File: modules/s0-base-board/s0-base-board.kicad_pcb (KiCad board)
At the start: 2 copper layers, 54.6 x 86.4 mm, 64 parts, among them J1 USB_C_Receptacle_USB2.0_14P, J2 Screw_Terminal_01x02, J3 BAT_JST_01x02, J4 RJ45_Bel_SI-60062-F JLC(C3467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, J5 Conn_02x23_Odd_Even, J6 Conn_02x23_Odd_Even, Q1 PMOS, U1 MCP73831-2-OT, U2 XL1509-5.0, U3 LM2575-3.3BU, U4 W5500, U5 NUP4202, Y1 25MHz

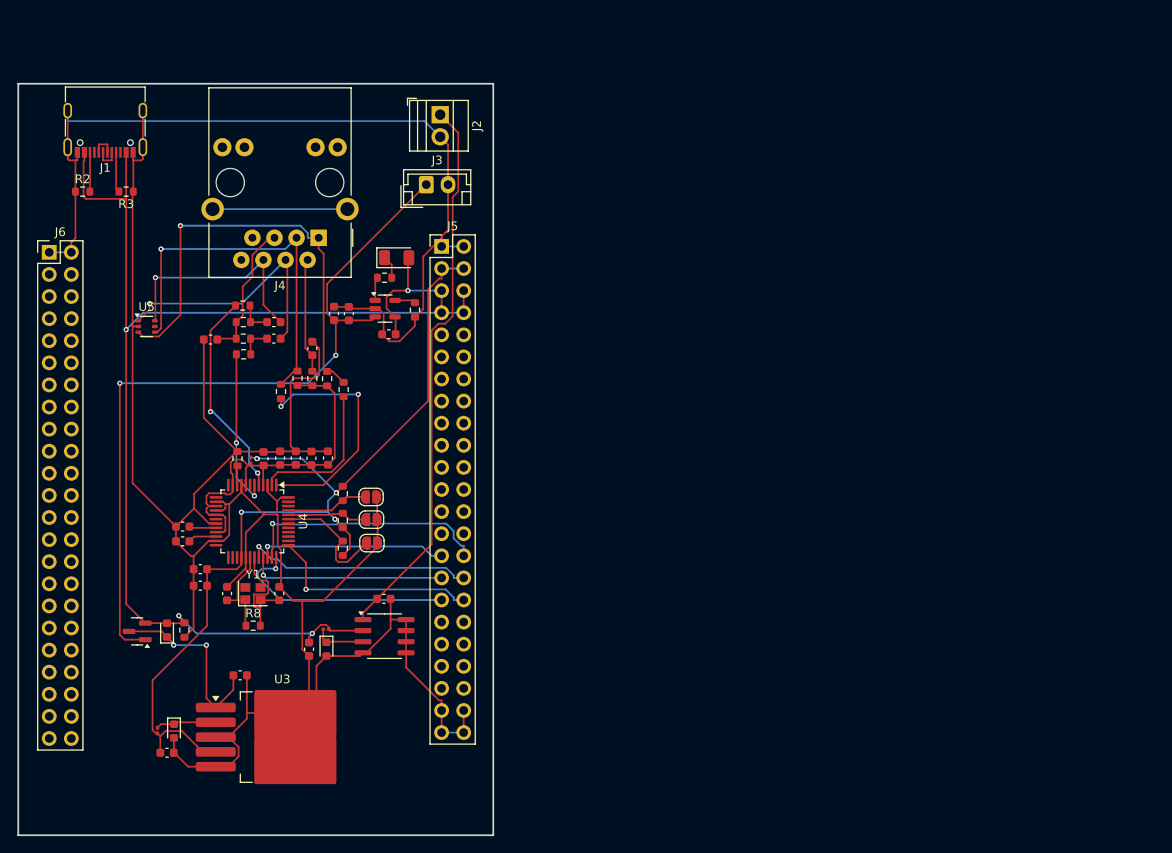
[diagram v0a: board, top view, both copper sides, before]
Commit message: Production build
Signed-off-by: Rodney Osodo <socials@rodneyosodo.com>
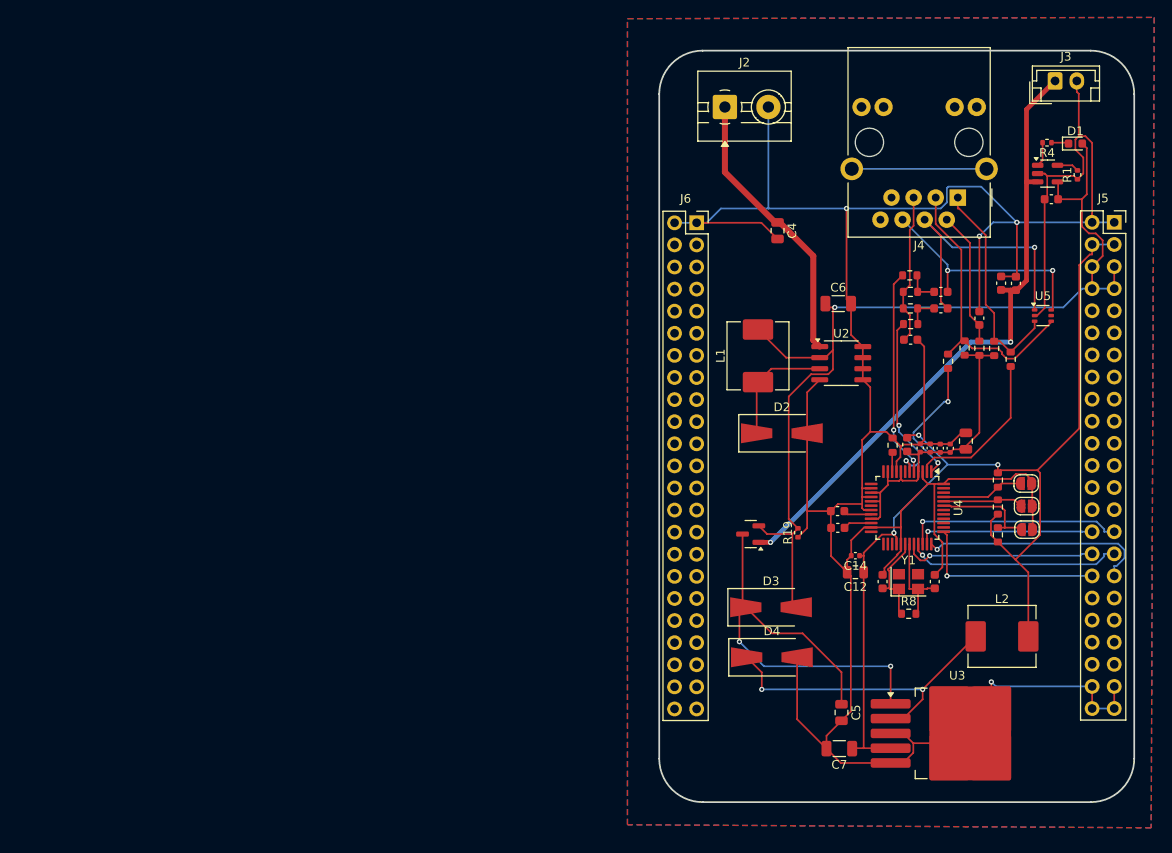
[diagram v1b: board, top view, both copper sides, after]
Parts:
- removed J1: USB_C_Receptacle_USB2.0_14P, Connector_USB:USB_C_Receptacle_G-Switch_GT-USB-7010ASV
- removed R2, R3: 5K1, Resistor_SMD:R_0603_1608Metric
- C10, C13, C14, C9: footprint Capacitor_SMD:C_0603_1608Metric -> Capacitor_SMD:C_0402_1005Metric
- C12: footprint Capacitor_SMD:C_0603_1608Metric -> Capacitor_SMD:C_0805_2012Metric
- C16: value 4.7uF -> 0.1uF; footprint Capacitor_SMD:C_0603_1608Metric -> Capacitor_SMD:C_0402_1005Metric
- C17: value 10nF -> 4.7uF
- C21: value 0.1uF -> 10uF; footprint Capacitor_SMD:C_0603_1608Metric -> Capacitor_SMD:C_0805_2012Metric
- C22: value 10uF -> 10nF
- C4, C5: value 680uF -> 10uF; footprint Capacitor_SMD:C_0603_1608Metric -> Capacitor_SMD:C_0805_2012Metric
- C6, C7: footprint Capacitor_SMD:C_0603_1608Metric -> Capacitor_SMD:C_1206_3216Metric
- D1: footprint LED_SMD:LED_1206_3216Metric -> LED_SMD:LED_0603_1608Metric
- D2, D3, D4: value D -> 40V 3A 550mV@3A Schottky; footprint Diode_SMD:D_0603_1608Metric -> Diode_SMD:D_SMA-SMB_Universal_Handsoldering
- J2: footprint TerminalBlock:TerminalBlock_Xinya_XY308-2.54-2P_1x02_P2.54mm_Horizontal -> TerminalBlock:TerminalBlock_MaiXu_MX126-5.0-02P_1x02_P5.00mm
- J4: value RJ45_Bel_SI-60062-F JLC(C34677) -> RJ45_Bel_SI-60062-F JLC
- J5, J6: footprint Connector_PinHeader_2.54mm:PinHeader_2x23_P2.54mm_Vertical -> Connector_PinSocket_2.54mm:PinSocket_2x23_P2.54mm_Vertical
- L1: value 68uH/2A -> 47uH/2A; footprint Inductor_SMD:L_0201_0603Metric -> Inductor_SMD:L_Chilisin_BMRB00060624
- L2: value 33uH -> 47uH/2A; footprint Inductor_SMD:L_0201_0603Metric -> Inductor_SMD:L_Chilisin_BMRB00060624
- L3: footprint Inductor_SMD:L_0201_0603Metric -> Inductor_SMD:L_0603_1608Metric
- R1, R19: footprint Resistor_SMD:R_0603_1608Metric -> Resistor_SMD:R_0402_1005Metric
- R4: value 2k -> 100; footprint Resistor_SMD:R_0603_1608Metric -> Resistor_SMD:R_0402_1005Metric
- R9: value 12.4K 1% -> 12K 1%
- U3: value LM2575-3.3BU -> LM2575S-3.3(UMW)
- Y1: footprint Crystal:Crystal_SMD_2520-4Pin_2.5x2.0mm -> Crystal:Crystal_SMD_3225-4Pin_3.2x2.5mm
- moved U5 103.0 mm to (202.6, 73.3)
- moved L2 97.7 mm to (197.9, 110.2), turned to 0 degrees
- moved C16 88.7 mm to (191.9, 88.5), turned to 90 degrees
- moved D1 79.1 mm to (206.3, 53.5)
- moved C1 77.7 mm to (203.6, 59.9)
- moved R4 77.7 mm to (203.1, 53.4)
- moved U1 77.7 mm to (203.1, 57.0)
- moved R1 77.7 mm to (206.6, 57.1)
- moved U3 77.6 mm to (192.8, 121.3)
- moved J5 77.4 mm to (210.8, 62.6)
- moved C7 77.3 mm to (179.2, 123.0), turned to 180 degrees
- moved C20 76.8 mm to (195.3, 73.6)
- moved C3 76.8 mm to (197.8, 69.5)
- moved R10 76.8 mm to (187.4, 74.2)
- moved R11 76.8 mm to (187.3, 68.7)
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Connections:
- C16 pad 1: Net-(U4-TOCAP) -> VCCA
- C17 pad 1: GND -> Net-(U4-TOCAP)
- C17 pad 2: Net-(J4-RCT) -> GND
- C22 pad 1: VCCA -> Net-(J4-RCT)
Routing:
- net +5V: track 154.6 -> 113.9 mm, vias 4 -> 1
- net Net-(D3-K): track 21.8 -> 53.5 mm
- net VIN: track 63.9 -> 32.4 mm
- net Net-(D4-K): track 6.96 -> 37.3 mm, vias 0 -> 2
- net Net-(J4-TD+): track 51.3 -> 25.4 mm, vias 1 -> 0
- net VBAT: track 87.9 -> 73.4 mm
- net +3V3: track 105.9 -> 120.1 mm, vias 4 -> 3
- net TXN: track 27.9 -> 15.2 mm
- net Net-(J4-TD-): track 44.0 -> 33.0 mm, vias 1 -> 0
- net MOSI: track 28.8 -> 20.4 mm
- net Net-(D2-K): track 5.85 -> 13.7 mm
- net VCCA: track 44.5 -> 38.8 mm
- net Net-(J1-CC1): track 4.64 -> 0.00 mm
- net Net-(J1-CC2): track 4.52 -> 0.00 mm
- net CS: track 26.5 -> 22.2 mm
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- added copper zone on B.Cu, net GND
- added copper zone on F.Cu, net GND
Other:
- outline, holes or cut-outs redrawn
